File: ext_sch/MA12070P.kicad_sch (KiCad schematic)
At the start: 49 parts

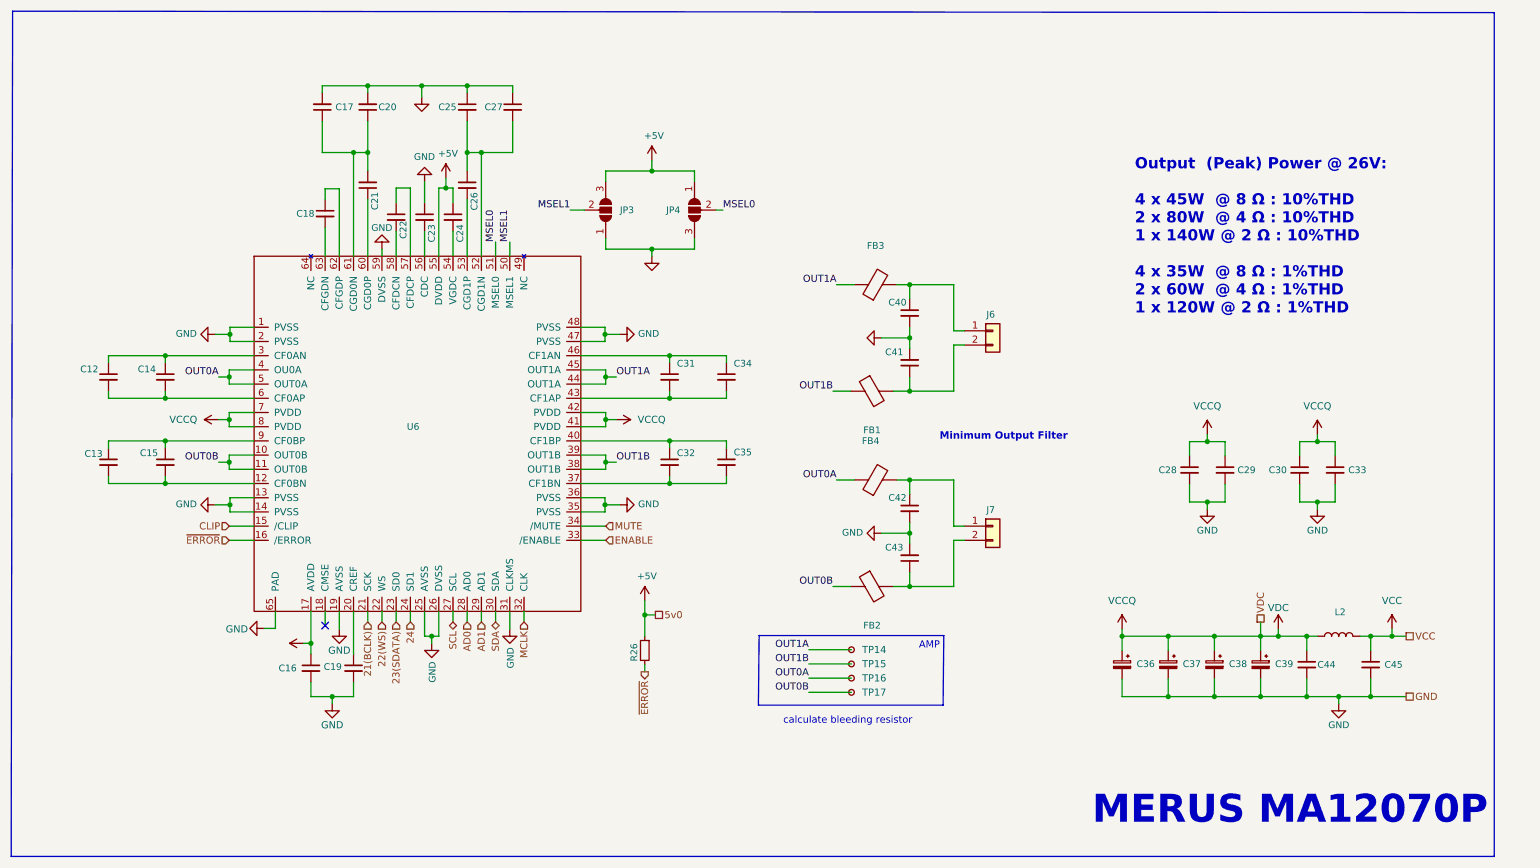
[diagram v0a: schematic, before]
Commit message: Updated readme and pictures!
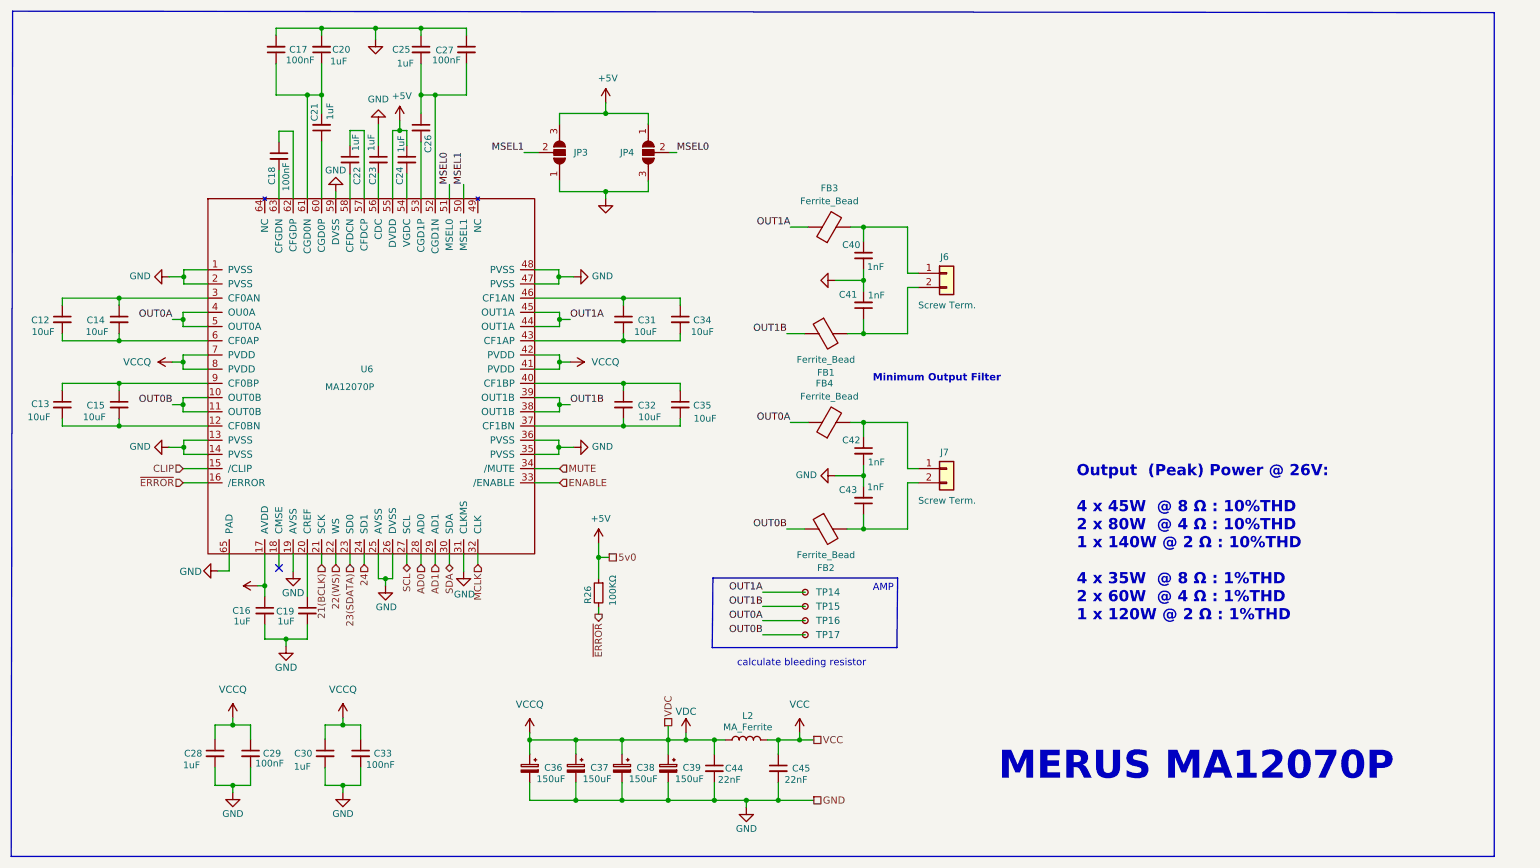
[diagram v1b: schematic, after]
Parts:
- C12, C13, C14, C15, C31, C32, C34, C35: value (none) -> 10uF; footprint (none) -> Capacitor_SMD:C_0805_2012Metric
- C16, C19, C21, C22, C23, C24, C26: value (none) -> 1uF; footprint (none) -> Capacitor_SMD:C_0603_1608Metric
- C17, C18, C27, C29, C33: value (none) -> 100nF; footprint (none) -> Capacitor_SMD:C_0603_1608Metric
- C20, C25, C28, C30: value (none) -> 1uF; footprint (none) -> Capacitor_SMD:C_0805_2012Metric
- C36, C37, C38, C39: value (none) -> 150uF; footprint (none) -> Capacitor_SMD:CP_Elec_8x10
- C40, C41, C42, C43: value (none) -> 1nF; footprint (none) -> Capacitor_SMD:C_0603_1608Metric
- C44, C45: value (none) -> 22nF; footprint (none) -> Capacitor_SMD:C_0603_1608Metric
- FB1, FB2, FB3, FB4: value (none) -> Ferrite_Bead; footprint (none) -> Capacitor_SMD:C_1206_3216Metric
- J6, J7: value (none) -> Screw Term.; footprint (none) -> Lib:Phoenix1989447
- JP3, JP4: value (none) -> Jumper_3_Bridged; footprint (none) -> Jumper:SolderJumper-3_P1.3mm_Bridged12_RoundedPad1.0x1.5mm
- L2: value (none) -> MA_Ferrite; footprint (none) -> Lib:MA_Ferrite
- R26: value (none) -> 100KΩ; footprint (none) -> Resistor_SMD:R_0603_1608Metric
- TP14, TP15, TP16, TP17: value (none) -> TestPoint_Small; footprint (none) -> TestPoint:TestPoint_Pad_D1.5mm
- U6: value (none) -> MA12070P; footprint (none) -> Package_DFN_QFN:QFN-64-1EP_9x9mm_P0.5mm_EP5.45x5.45mm_ThermalVias
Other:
- moved on the sheet: C12, C13, C14, C15, C16, C17, C18, C19, C20, C21, C22, C23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
